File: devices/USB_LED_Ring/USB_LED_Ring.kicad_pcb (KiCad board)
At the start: 2 copper layers, 93.5 x 75 mm, 87 parts, among them J1 JST SH 3 Vert, J2 USB_B_Micro, J3 JST SH 3 Vert, J4 .100, Q1 DMG2305UX, U1 TPS923610, U2 TLV75733PDBV, U3 RP2354A, Y1 ABM8-272-T3

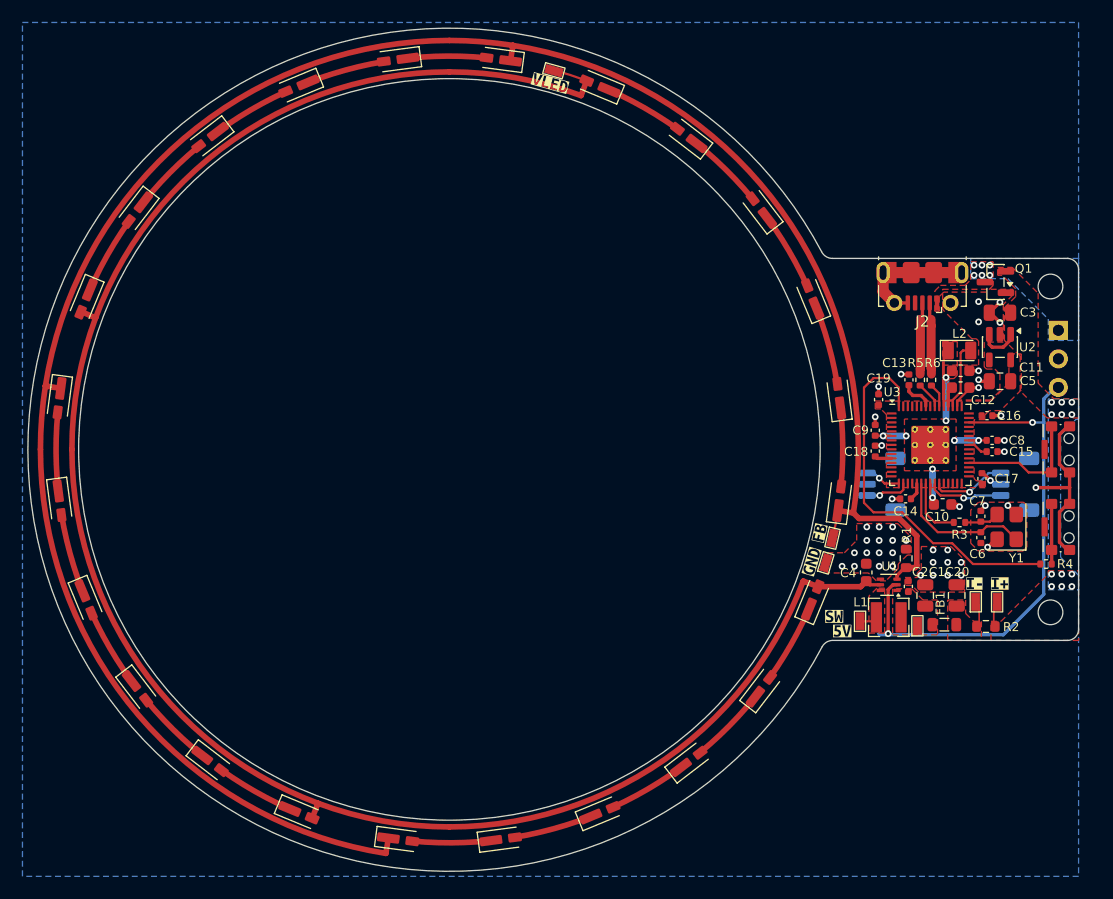
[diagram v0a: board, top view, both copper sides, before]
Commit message: !fixup
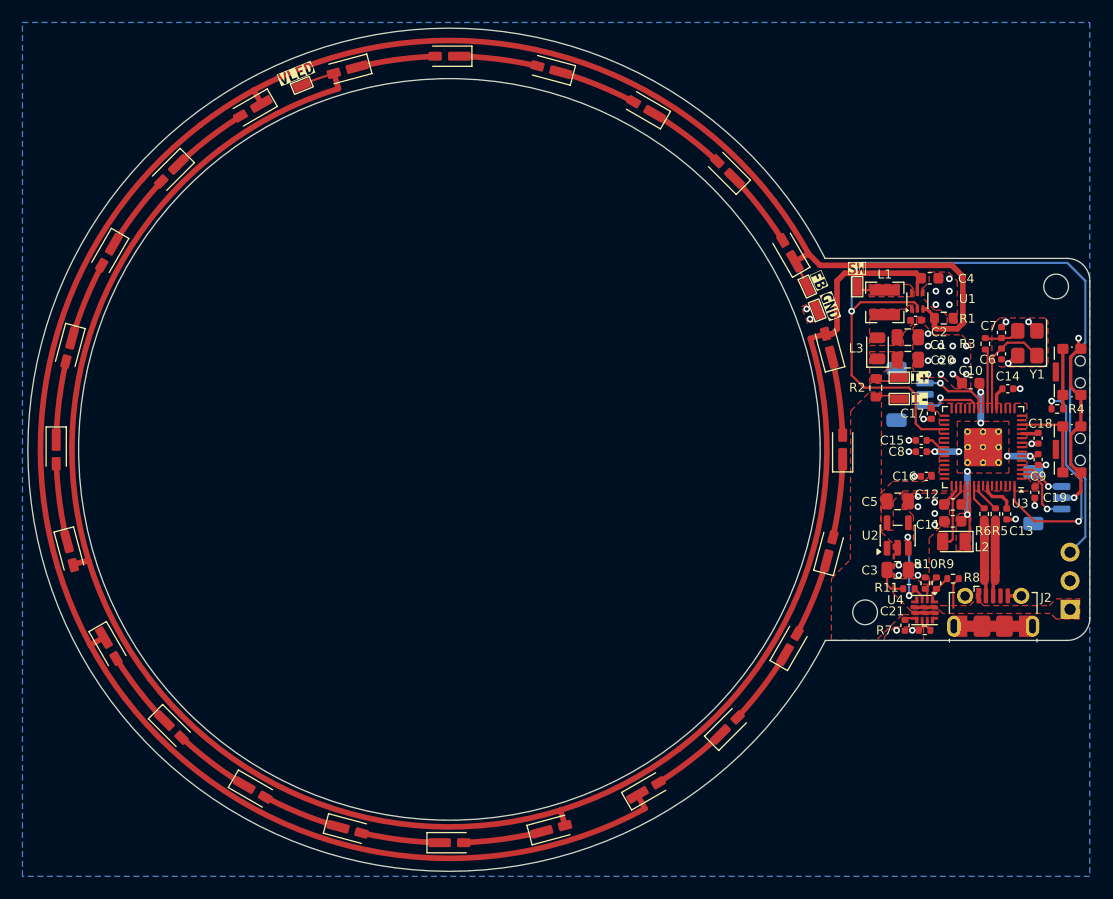
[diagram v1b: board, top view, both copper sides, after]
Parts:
- removed FB1: MLZ2012DR22DT000, Inductor_SMD:L_0805_2012Metric
- removed Q1: DMG2305UX, Package_TO_SOT_SMD:SOT-23
- removed TP7: RCUCTE, custom:RCUCTE
- removed kibuzzard-6A15B62E: G***, kibuzzard-6A15B62E
- added C21: 1n, Capacitor_SMD:C_0402_1005Metric, F.Cu at (190.6, 115.7)
- added L3: 220n, LED_SMD:LED_0805_2012Metric, F.Cu at (188.1, 91.0)
- added R10: 130k, Resistor_SMD:R_0402_1005Metric, F.Cu at (192.3, 111.9)
- added R11: 47k, Resistor_SMD:R_0402_1005Metric, F.Cu at (190.9, 112.4)
- added R7: 6k8, Resistor_SMD:R_0402_1005Metric, F.Cu at (192.3, 116.1)
- added R8: 430k, Resistor_SMD:R_0402_1005Metric, F.Cu at (194.8, 111.5)
- added R9: 47k, Resistor_SMD:R_0402_1005Metric, F.Cu at (193.3, 111.9)
- added U4: TPS25947xx, custom:Texas_RPW_VQFN-HR-10_2.1x2.1mm_P0.475mm, F.Cu at (192.3, 114.3)
- C20: value 2u2 -> 4u7
- R2: value 150m -> 100m
- moved kibuzzard-6A15B584 31.0 mm to (186.3, 83.9)
- moved TP1 29.8 mm to (186.3, 85.5)
- moved J2 29.7 mm to (198.4, 114.5), turned to 0 degrees
- moved L1 28.0 mm to (188.8, 86.9), turned to 90 degrees
- moved C4 26.8 mm to (192.8, 84.8), turned to 0 degrees
- moved U1 25.4 mm to (191.7, 86.8), turned to 90 degrees
- moved J4 24.9 mm to (205.2, 114.2), turned to 0 degrees
- moved kibuzzard-69FB6775 24.7 mm to (202.6, 114.1)
- moved C3 24.6 mm to (189.9, 110.7), turned to 0 degrees
- moved C2 23.7 mm to (191.5, 88.5), turned to 0 degrees
- moved R2 23.4 mm to (187.9, 94.5), turned to 90 degrees
- moved C1 23.0 mm to (190.8, 90.0), turned to 0 degrees
- moved kibuzzard-6A15B5C8 22.8 mm to (183.9, 87.2), turned to -69.27 degrees
- moved kibuzzard-6A15B60A 22.6 mm to (136.3, 66.5), turned to 22.08 degrees
- moved D12 22.5 mm to (167.5, 130.3), turned to -150 degrees
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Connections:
- U2 pad 3: VIN -> /RUN
- U3 pad 13: unconnected-(U3-GPIO9-Pad13) -> /BTN
- U3 pad 16: /UART_TX -> unconnected-(U3-GPIO12-Pad16)
- U3 pad 17: /UART_RX -> unconnected-(U3-GPIO13-Pad17)
- U3 pad 2: unconnected-(U3-GPIO0-Pad2) -> /UART_TX
- U3 pad 3: unconnected-(U3-GPIO1-Pad3) -> /UART_RX
- U3 pad 34: /BTN -> /LED_PWM
- U3 pad 43: /LED_PWM -> unconnected-(U3-GPIO29_ADC3-Pad43)
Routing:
- net /LED_PWM: track 46.9 -> 75.1 mm, vias 2 -> 1
- net /BTSEL: track 33.7 -> 20.9 mm, vias 0 -> 2
- net /LED_FB: track 11.6 -> 23.7 mm
- net /VLED: track 5.88 -> 14.8 mm
- net /RUN: track 0.00 -> 8.39 mm, vias 0 -> 2
- net GND: track 44.2 -> 38.9 mm
- net /BTN: track 11.8 -> 7.82 mm
- net /XIN: track 12.6 -> 9.53 mm
- net VBUS: track 0.00 -> 2.80 mm, vias 6 -> 0
- net /UART_TX: track 3.21 -> 5.85 mm
- net /OVLO: track 0.00 -> 2.50 mm
- net /UVLO: track 0.00 -> 2.48 mm
- net /SWDIO: track 6.77 -> 5.63 mm
- net /ILIM: track 0.00 -> 1.02 mm
- net /SW: track 1.59 -> 2.57 mm
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- removed copper zone on B.Cu, net VBUS
- removed copper zone on B.Cu, net VIN
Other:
- board size 93.5 x 75 mm -> 94.5 x 75 mm
